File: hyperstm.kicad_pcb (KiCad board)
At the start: 2 copper layers, 38.1 x 38.1 mm, 2 parts, among them J1 Conn_01x12, U1 S27KL0641

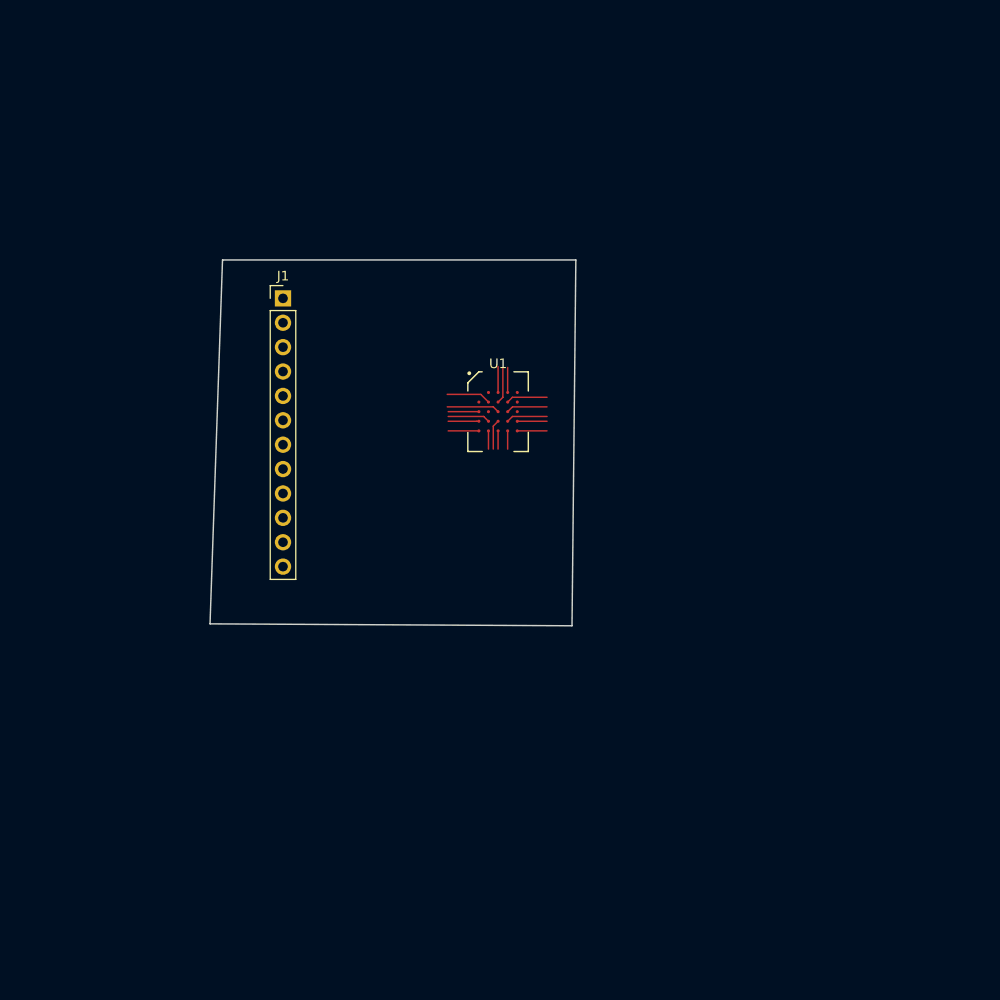
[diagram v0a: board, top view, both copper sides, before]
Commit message: More work
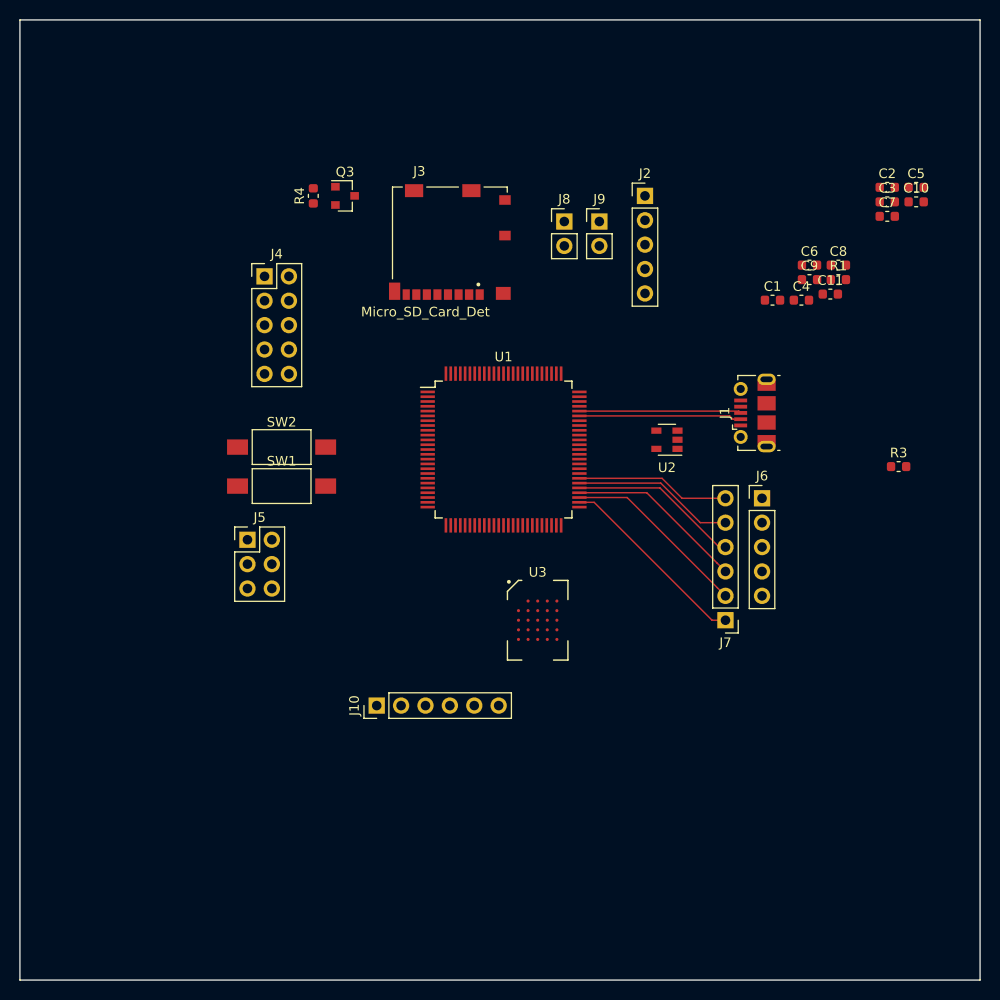
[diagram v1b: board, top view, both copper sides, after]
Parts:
- added C1: 10uF, Capacitor_SMD:C_0603_1608Metric, F.Cu at (178.4, 79.2)
- added C10: 100nF, Capacitor_SMD:C_0603_1608Metric, F.Cu at (193.3, 68.9)
- added C11: 1uF, Capacitor_SMD:C_0603_1608Metric, F.Cu at (184.4, 78.6)
- added C2: 100nF, Capacitor_SMD:C_0603_1608Metric, F.Cu at (190.3, 67.4)
- added C3: 100nF, Capacitor_SMD:C_0603_1608Metric, F.Cu at (190.3, 68.9)
- added C4: 100nF, Capacitor_SMD:C_0603_1608Metric, F.Cu at (181.4, 79.2)
- added C5: 100nF, Capacitor_SMD:C_0603_1608Metric, F.Cu at (193.3, 67.4)
- added C6: 100nF, Capacitor_SMD:C_0603_1608Metric, F.Cu at (182.2, 75.5)
- added C7: 100nF, Capacitor_SMD:C_0603_1608Metric, F.Cu at (190.3, 70.5)
- added C8: 100nF, Capacitor_SMD:C_0603_1608Metric, F.Cu at (185.2, 75.5)
- added C9: 100nF, Capacitor_SMD:C_0603_1608Metric, F.Cu at (182.2, 77.0)
- added J10: SPI1, Connector_PinHeader_2.54mm:PinHeader_1x06_P2.54mm_Vertical, F.Cu at (137.2, 121.4)
- added J2: DBG_HEADER, Connector_PinHeader_2.54mm:PinHeader_1x05_P2.54mm_Vertical, F.Cu at (165.1, 68.3)
- added J3: Micro_SD_Card_Det, Molex_SDCARD:MOLEX_104031-0811, F.Cu at (144.8, 73.4)
- added J4: Analog_Header, Connector_PinHeader_2.54mm:PinHeader_2x05_P2.54mm_Vertical, F.Cu at (125.5, 76.7)
- added J5: UART_COMBO, Connector_PinHeader_2.54mm:PinHeader_2x03_P2.54mm_Vertical, F.Cu at (123.7, 104.1)
- added J6: USART1, Connector_PinHeader_2.54mm:PinHeader_1x05_P2.54mm_Vertical, F.Cu at (177.3, 99.8)
- added J7: SPI2, Connector_PinHeader_2.54mm:PinHeader_1x06_P2.54mm_Vertical, F.Cu at (173.5, 112.5)
- added J8: I2C1, Connector_PinHeader_2.54mm:PinHeader_1x02_P2.54mm_Vertical, F.Cu at (156.7, 71.0)
- added J9: I2C4, Connector_PinHeader_2.54mm:PinHeader_1x02_P2.54mm_Vertical, F.Cu at (160.3, 71.0)
- added Q3: FDN340P, Package_TO_SOT_SMD:SOT-23, F.Cu at (133.9, 68.3)
- added R1: 10k, Resistor_SMD:R_0603_1608Metric, F.Cu at (185.2, 77.0)
- added R3: 10k, Resistor_SMD:R_0603_1608Metric, F.Cu at (191.5, 96.5)
- added R4: 1k, Resistor_SMD:R_0603_1608Metric, F.Cu at (130.6, 68.3)
- added SW1: SW_SPST, Button_Switch_SMD:SW_SPST_FSMSM, F.Cu at (127.3, 98.6)
- added SW2: SW_SPST, Button_Switch_SMD:SW_SPST_FSMSM, F.Cu at (127.3, 94.5)
- added U2: MIC5219-3.3, Package_TO_SOT_SMD:SOT-23-5, F.Cu at (167.4, 93.7)
- added U3: S27KL0641, BGA_Extra:BGA-25_5x5_6.0x8.0mm, F.Cu at (153.9, 112.5)
- J1: value Conn_01x12 -> USB_B_Micro; footprint Connector_PinHeader_2.54mm:PinHeader_1x12_P2.54mm_Vertical -> Connector_USB:USB_Micro-B_Molex-105017-0001
- U1: value S27KL0641 -> STM32L4R5VITx; footprint BGA_Extra:BGA-25_5x5_6.0x8.0mm -> Package_QFP:LQFP-100_14x14mm_P0.5mm
- moved J1 50.6 mm to (176.5, 90.9), turned to 90 degrees
- moved U1 3.98 mm to (150.4, 94.7)
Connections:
- J1 pad 1: /~RESET~ -> Net-(J1-Pad1)
- J1 pad 2: /RWDS -> /Microcontroller/USB_D-
- J1 pad 3: /DQ7 -> /Microcontroller/USB_D+
- J1 pad 4: /DQ6 -> Net-(J1-Pad4)
- J1 pad 5: /DQ5 -> GND
- J1 pad 6: /DQ4 -> GND
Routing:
- net /Microcontroller/SPI2_SCK: track 0.00 -> 20.3 mm
- net /Microcontroller/SPI2_MISO: track 0.00 -> 19.5 mm
- net /Microcontroller/SPI2_MOSI: track 0.00 -> 18.6 mm
- net /Microcontroller/SPI2_CS1: track 0.00 -> 17.8 mm
- net /Microcontroller/USB_D-: track 0.00 -> 16.9 mm
- net /Microcontroller/SPI2_CS2: track 0.00 -> 16.9 mm
- net /Microcontroller/USB_D+: track 0.00 -> 16.9 mm
- net /Microcontroller/SPI2_CS3: track 0.00 -> 16.1 mm
- net GND: track 10.1 -> 0.00 mm
- net VDD: track 9.41 -> 0.00 mm
- net /RWDS: track 5.51 -> 0.00 mm
- net /CK: track 4.63 -> 0.00 mm
- net /DQ1: track 4.41 -> 0.00 mm
- net /DQ3: track 4.31 -> 0.00 mm
- net /DQ2: track 4.31 -> 0.00 mm
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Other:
- board size 38.1 x 38.1 mm -> 100 x 100 mm

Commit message: More updates
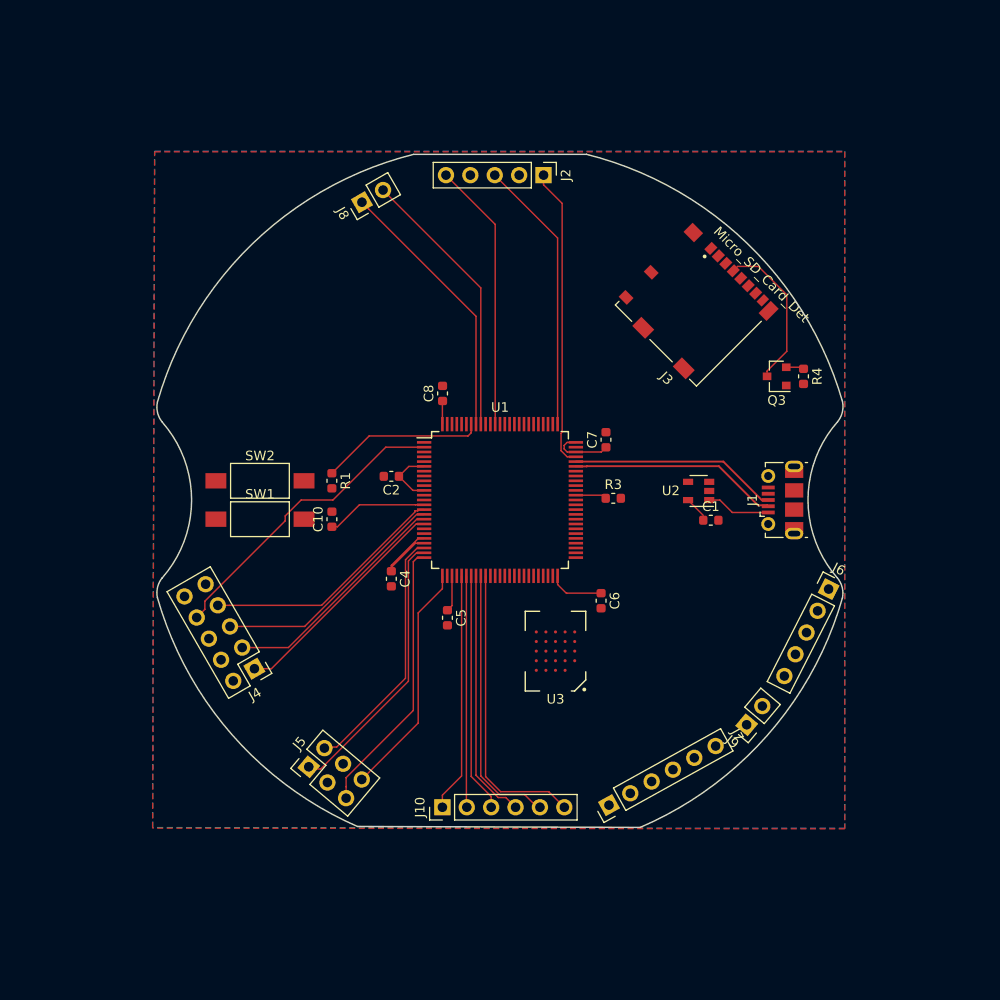
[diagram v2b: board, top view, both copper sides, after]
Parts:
- removed C11: 1uF, Capacitor_SMD:C_0603_1608Metric
- removed C3, C9: 100nF, Capacitor_SMD:C_0603_1608Metric
- moved C10 69.2 mm to (132.5, 102.0), turned to 90 degrees
- moved C5 66.3 mm to (144.5, 112.3), turned to 270 degrees
- moved C2 59.8 mm to (138.7, 97.5), turned to 180 degrees
- moved R1 56.8 mm to (132.5, 98.0), turned to 270 degrees
- moved J9 54.6 mm to (175.7, 123.4), turned to 140 degrees
- moved R4 54.4 mm to (181.6, 87.1), turned to 270 degrees
- moved C4 51.6 mm to (138.7, 108.2), turned to 270 degrees
- moved Q3 48.7 mm to (178.8, 87.1), turned to 180 degrees
- moved C8 43.3 mm to (144.0, 88.9), turned to 90 degrees
- moved C6 41.1 mm to (160.5, 110.5), turned to 270 degrees
- moved J4 40.9 mm to (124.4, 117.6), turned to 210 degrees
- moved C7 37.4 mm to (161.0, 93.7), turned to 90 degrees
- moved R3 29.9 mm to (161.8, 99.8)
- moved J3 26.5 mm to (170.5, 79.7), turned to 135 degrees
- moved J5 24.5 mm to (130.1, 127.8), turned to 50 degrees
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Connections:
- net Net-(J1-Pad1) renamed /Microcontroller/VBUS
- J4 pad 10: /Microcontroller/TIM1_CH1 -> GND
- J4 pad 2: /Microcontroller/ADC1_IN3 -> /Microcontroller/TIM1_CH1
- J4 pad 3: /Microcontroller/ADC1_IN2 -> /Microcontroller/ADC1_IN3
- J4 pad 4: /Microcontroller/ADC1_IN -> /Microcontroller/TIM1_CH2
- J4 pad 5: GND -> /Microcontroller/ADC1_IN2
- J4 pad 6: GND -> /Microcontroller/TIM2_CH1
- J4 pad 7: /Microcontroller/TIM3_CH1 -> /Microcontroller/ADC1_IN
- J4 pad 8: /Microcontroller/TIM2_CH1 -> /Microcontroller/TIM3_CH1
- J4 pad 9: /Microcontroller/TIM1_CH2 -> GND
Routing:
- net +3V3: track 0.00 -> 38.9 mm
- net /Microcontroller/TIM3_CH1: track 0.00 -> 31.8 mm
- net /Microcontroller/SWDIO: track 0.00 -> 31.3 mm
- net /Microcontroller/SPI1_CS3: track 0.00 -> 30.4 mm
- net /Microcontroller/LPUART1_TX: track 0.00 -> 28.8 mm
- net /Microcontroller/UART4_RX: track 0.00 -> 28.8 mm
- net /Microcontroller/SWCLK: track 0.00 -> 28.6 mm
- net /Microcontroller/I2C1_SCL: track 0.00 -> 28.6 mm
- net /Microcontroller/SPI1_CS2: track 0.00 -> 28.3 mm
- net /Microcontroller/SWO: track 0.00 -> 28.1 mm
- net /Microcontroller/I2C1_SDA: track 0.00 -> 28.0 mm
- net /Microcontroller/UART4_TX: track 0.00 -> 26.3 mm
- net /Microcontroller/SPI1_CS1: track 0.00 -> 26.3 mm
- net /Microcontroller/ADC1_IN: track 0.00 -> 25.7 mm
- net /Microcontroller/ADC1_IN2: track 0.00 -> 25.1 mm
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- added copper zone on B.Cu, net GND
- added copper zone on F.Cu, net GND
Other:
- board size 100 x 100 mm -> 71.5 x 70.1 mm
